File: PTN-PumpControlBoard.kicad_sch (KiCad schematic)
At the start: 10 parts, among them J1 PeripheralCANConnector, U1 EMC2305-1-AP-TR, U2 PeripheralSOM, U3 ST7735R

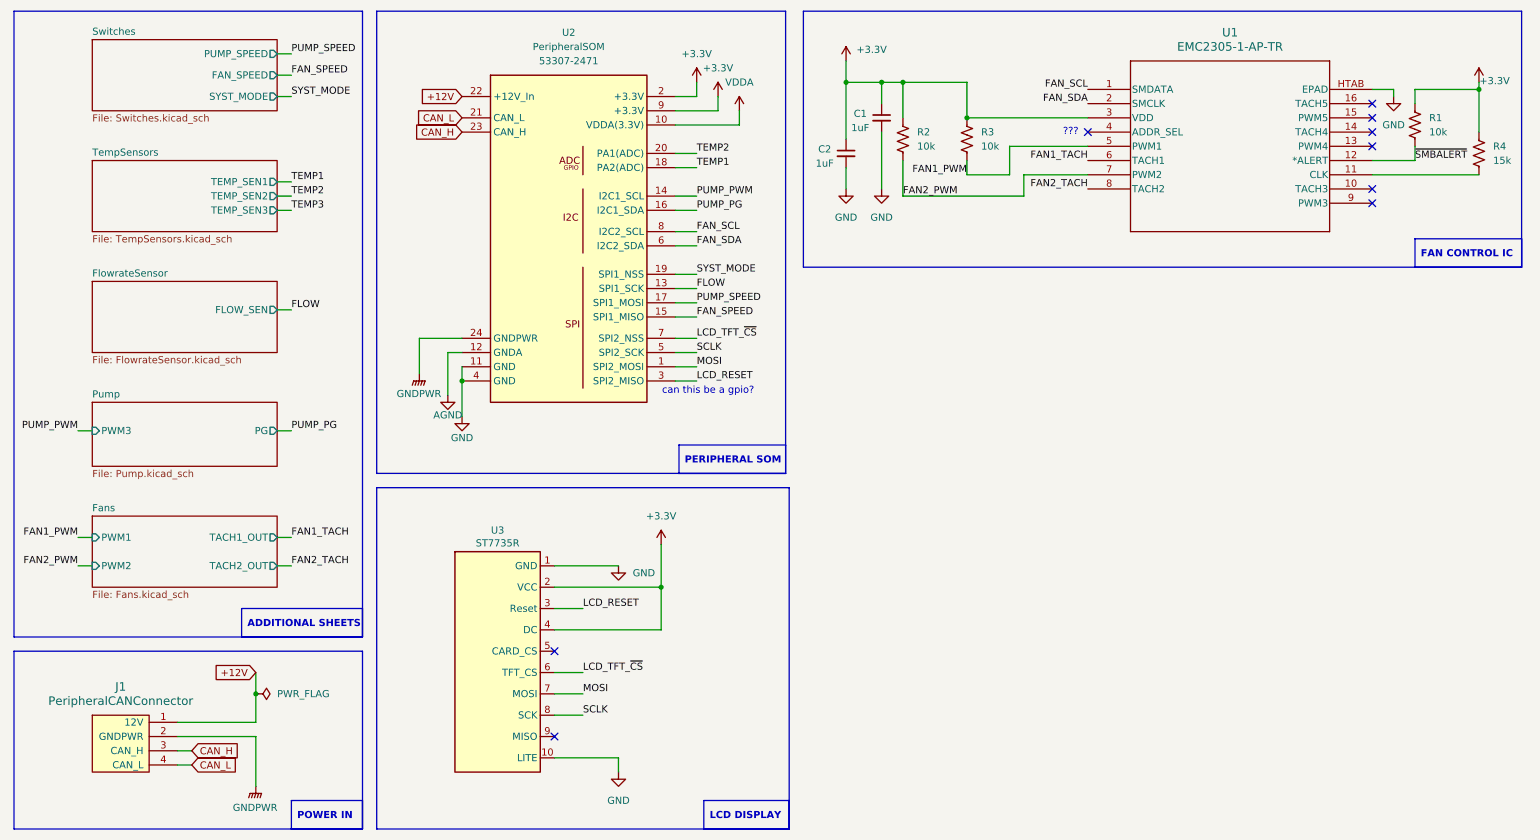
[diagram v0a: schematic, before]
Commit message: schematic with 12V components, unigain buffers & extra temp sensor
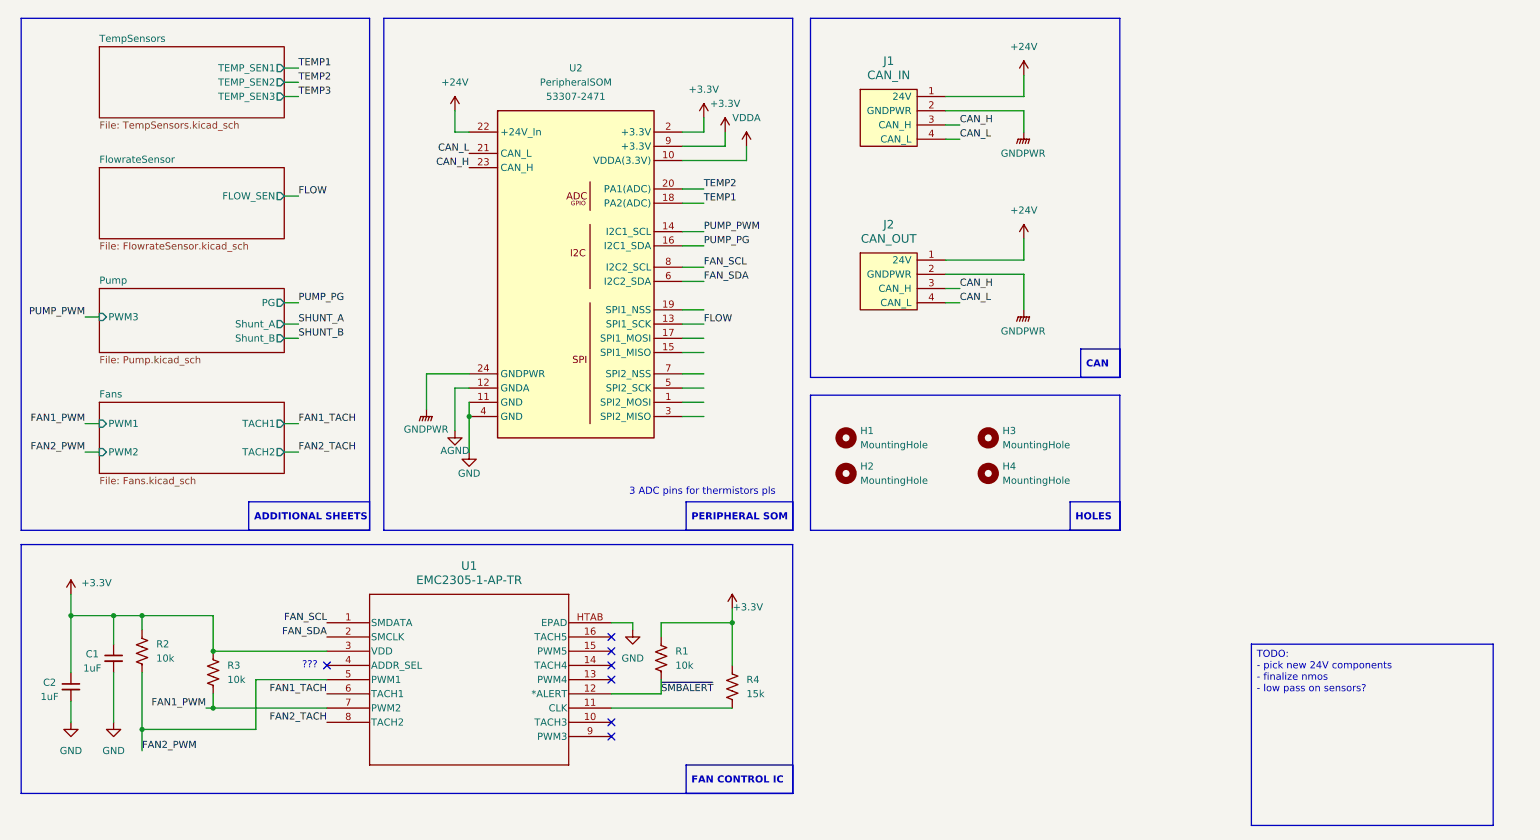
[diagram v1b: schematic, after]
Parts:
- removed U3: ST7735R, LCD:adafruit_st7735r, symbol Misc:ST7735
- added H1, H2, H3, H4: MountingHole, MountingHole:MountingHole_3.2mm_M3, symbol Mechanical:MountingHole
- added J2: CAN_OUT, Connector_Molex:Molex_Nano-Fit_105309-xx04_1x04_P2.50mm_Vertical, symbol utsvt-connectors:PeripheralCANConnector
- J1: value PeripheralCANConnector -> CAN_IN; footprint UTSVT_Connectors:Molex_MicroFit3.0_1x4xP3.00mm_PolarizingPeg_Vertical -> Connector_Molex:Molex_Nano-Fit_105309-xx04_1x04_P2.50mm_Vertical
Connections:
- net CAN_H: now also J2.3 (CAN_H)
- net CAN_L: now also J2.4 (CAN_L)
- net FAN1_PWM: now also U1.7 (PWM2); no longer U1.5 (PWM1)
- net FAN2_PWM: now also U1.5 (PWM1); no longer U1.7 (PWM2)
- net GNDPWR: now also J2.2 (GNDPWR)
- net +12V renamed +24V
- net +24V: now also J2.1 (24V)
- net FAN_SPEED: no longer names the net of U2.15 (SPI1_MISO)
- net LCD_RESET: no longer names the net of U2.3 (SPI2_MISO)
- net LCD_TFT_~{CS}: no longer names the net of U2.7 (SPI2_NSS)
- net MOSI: no longer names the net of U2.1 (SPI2_MOSI)
- net PUMP_SPEED: no longer names the net of U2.17 (SPI1_MOSI)
- net SCLK: no longer names the net of U2.5 (SPI2_SCK)
- net SYST_MODE: no longer names the net of U2.19 (SPI1_NSS)
- no-connect marks 9 -> 7
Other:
- removed sheet Switches
- sheet Fans ports: added TACH1, TACH2; removed TACH1_OUT, TACH2_OUT
- sheet Pump ports: added Shunt_A, Shunt_B; removed none
- note added: "3 ADC pins for thermistors pls"
- note removed: "can this be a gpio?"
- moved on the sheet: C1, C2, J1, R1, R2, R3, R4, U1, U2
